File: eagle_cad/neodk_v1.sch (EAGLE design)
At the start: 73 parts, among them J1 SWD, J2 Power 5V..12V DC, J3 FC68131, J4 S2B-XH-A(LF)(SN), J5 S2B-XH-A(LF)(SN), Q1 IRLML6344TRPBF, Q2 IRLML6344TRPBF, Q3 PMV50EPEAR, SW2 FSMRA6JH, U1 SGM61410XN6G/TR, U2 INA180A1IDBVR, U3 STM32G071KBT6, U4 VOT8024AM-T, U5 VOT8024AM-T, U6 VOT8024AM-T, U7 VOT8024AM-T, U8 AP63203, Y1 32.768 kHz

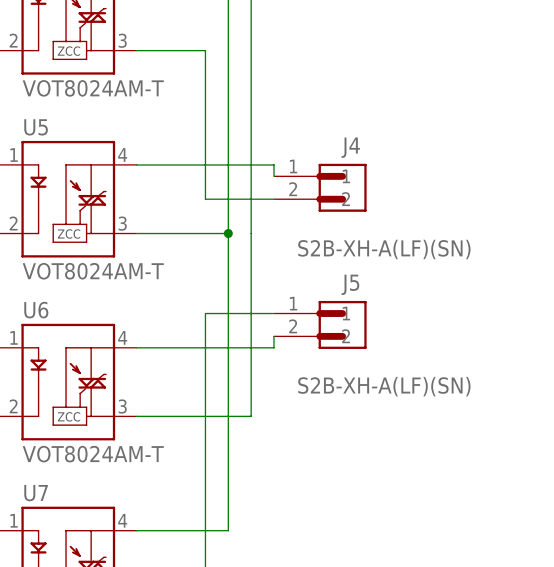
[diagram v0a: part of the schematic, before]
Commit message: More firmware and Eagle board file.
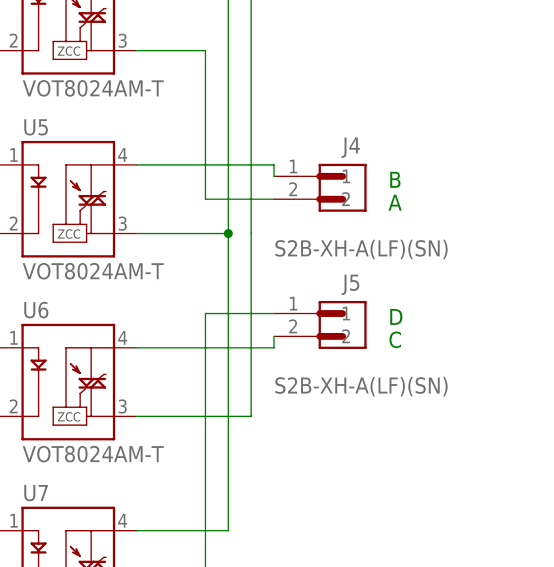
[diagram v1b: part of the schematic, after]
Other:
- note added: "A"
- note added: "B"
- note added: "C"
- note added: "D"
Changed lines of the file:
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@@
 <text x="88.9" y="-25.4" size="1.778" layer="91">TX</text>
 <text x="88.9" y="-27.94" size="1.778" layer="91">RX</text>
+<text x="228.6" y="-25.4" size="1.778" layer="91">A</text>
+<text x="228.6" y="-22.86" size="1.778" layer="91">B</text>
+<text x="228.6" y="-40.64" size="1.778" layer="91">C</text>
+<text x="228.6" y="-38.1" size="1.778" layer="91">D</text>
 </plain>
 <instances>
@@
 <instance part="J4" gate="G$1" x="223.52" y="-22.86" smashed="yes">
 <attribute name="NAME" x="223.52" y="-19.05" size="1.778" layer="95"/>
-<attribute name="VALUE" x="218.44" y="-30.48" size="1.778" layer="96"/>
+<attribute name="VALUE" x="215.9" y="-30.48" size="1.778" layer="96"/>
 </instance>
 <instance part="J5" gate="G$1" x="223.52" y="-38.1" smashed="yes">
 <attribute name="NAME" x="223.52" y="-34.29" size="1.778" layer="95"/>
-<attribute name="VALUE" x="218.44" y="-45.72" size="1.778" layer="96"/>
+<attribute name="VALUE" x="215.9" y="-45.72" size="1.778" layer="96"/>
 </instance>
 <instance part="D3" gate="G$1" x="25.4" y="-30.48" smashed="yes" rot="R90">
